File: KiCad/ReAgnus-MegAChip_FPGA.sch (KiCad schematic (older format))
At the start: 2 parts, among them U7 GW1N-UV9LQ144

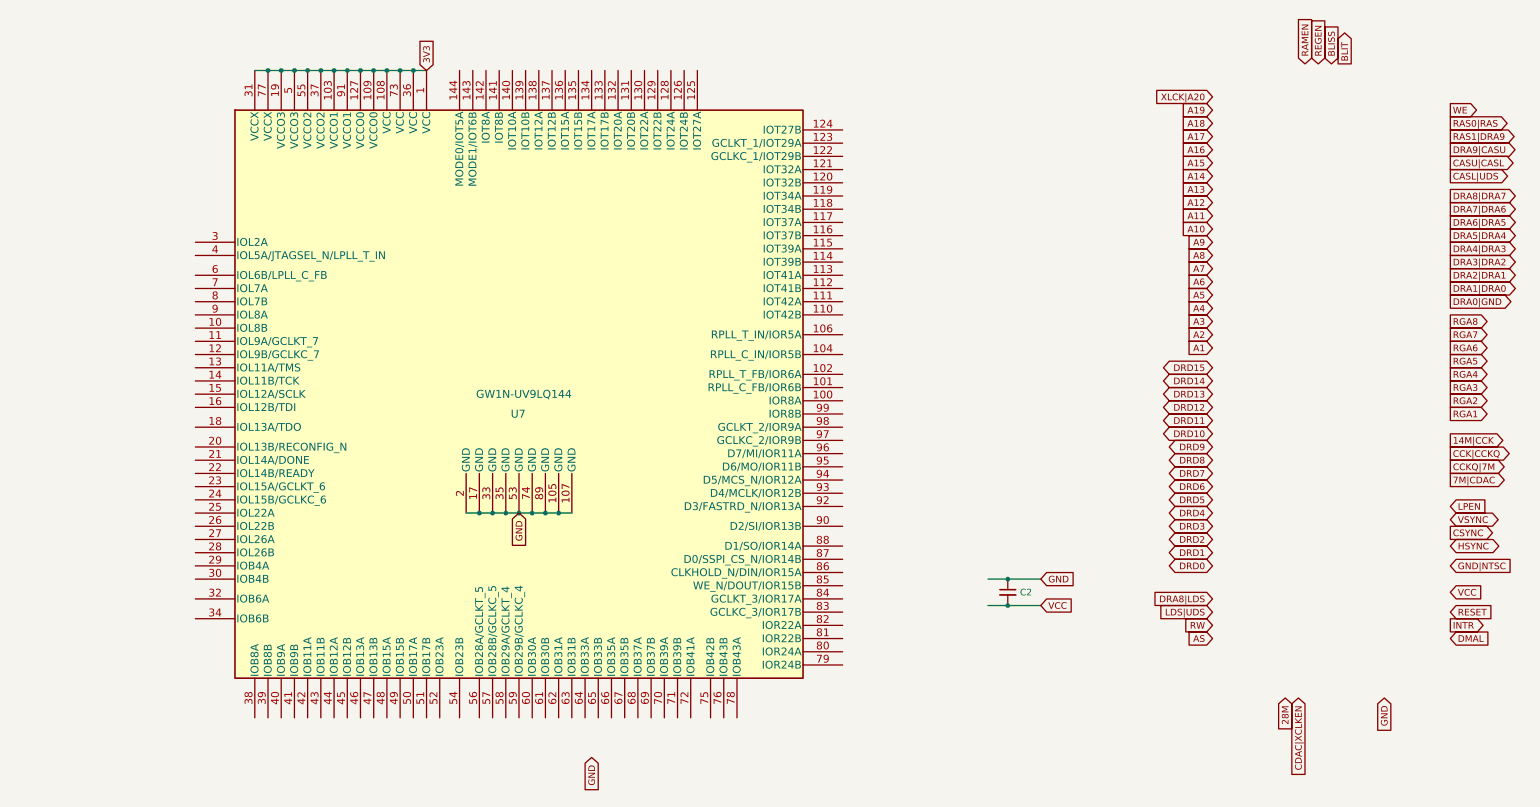
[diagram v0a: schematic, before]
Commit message: more routing and placing components
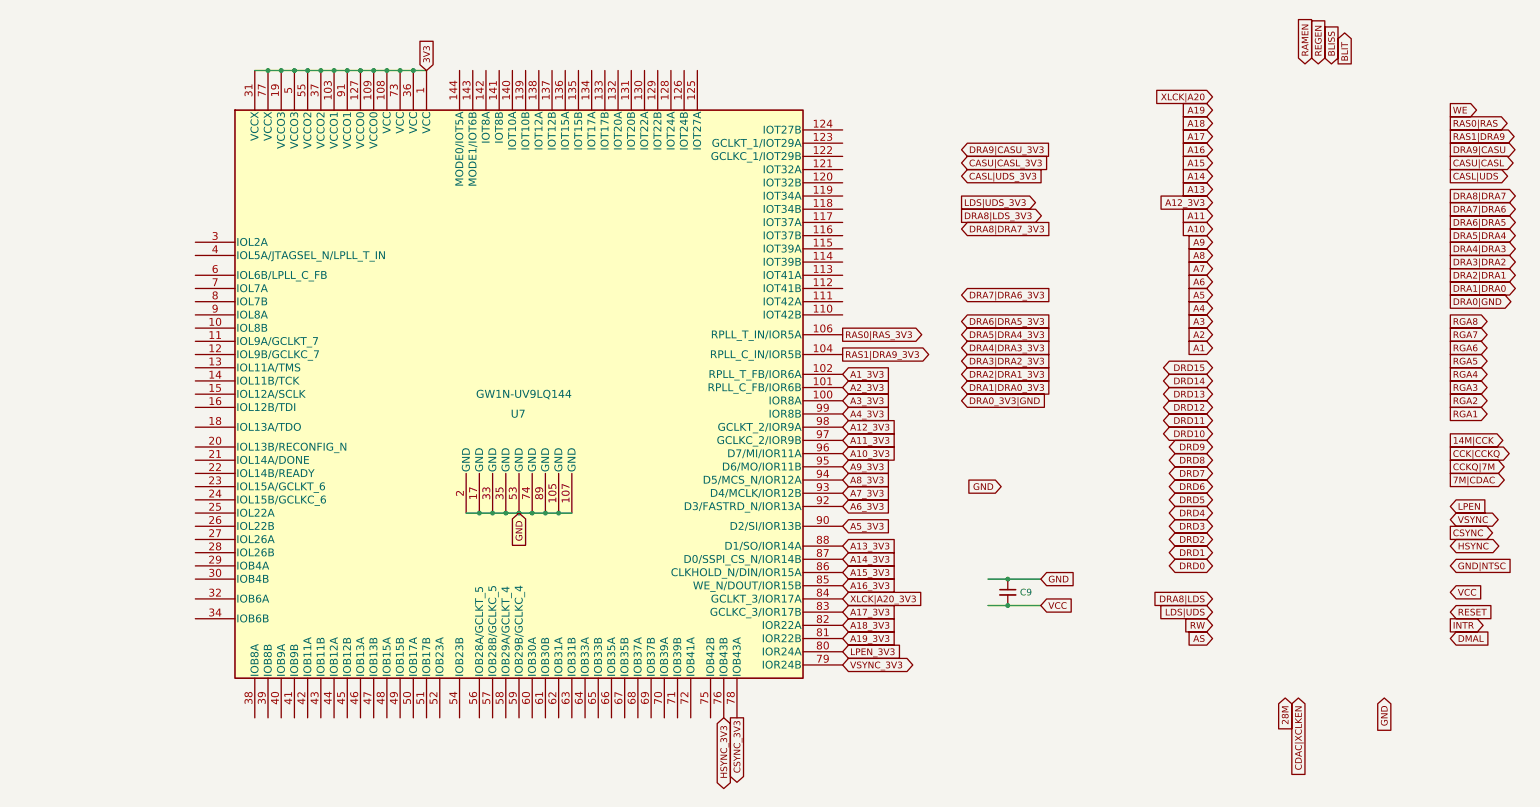
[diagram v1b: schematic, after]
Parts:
- U7: footprint Package_QFP:EQFP-144-1EP_20x20mm_P0.5mm_EP5x5mm -> Package_QFP:LQFP-144_20x20mm_P0.5mm
- renumbered C2 to C9
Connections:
- net labels added: A10_3V3, A11_3V3, A12_3V3, A13_3V3, A14_3V3, A15_3V3, A16_3V3, A17_3V3, A18_3V3, A19_3V3, A1_3V3, A2_3V3, A3_3V3, A4_3V3, A5_3V3, A6_3V3, A7_3V3, A8_3V3, A9_3V3, CASL|UDS_3V3, CASU|CASL_3V3, CSYNC_3V3, DRA0_3V3|GND, DRA1|DRA0_3V3, DRA2|DRA1_3V3, DRA3|DRA2_3V3, DRA4|DRA3_3V3, DRA5|DRA4_3V3, DRA6|DRA5_3V3, DRA7|DRA6_3V3, DRA8|DRA7_3V3, DRA8|LDS_3V3, DRA9|CASU_3V3, HSYNC_3V3, LDS|UDS_3V3, LPEN_3V3, RAS0|RAS_3V3, RAS1|DRA9_3V3, VSYNC_3V3, XLCK|A20_3V3
- net labels removed: A12
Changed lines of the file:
@@
 Comment4 ""
 $EndDescr
-Text GLabel 3900 6350 3    50   Input ~ 0
+Text GLabel 7000 4300 0    50   Input ~ 0
 GND
 Text GLabel 7300 5200 2    50   Input ~ 0
@@
 AR Path="/632F85C6" Ref="C?"  Part="1"
 AR Path="/632D3BDF/632F85C6" Ref="C?"  Part="1"
-AR Path="/632F104D/632F85C6" Ref="C2"  Part="1"
-F 0 "C2" H 7142 5100 50  0000 L CNN
+AR Path="/632F104D/632F85C6" Ref="C9"  Part="1"
+F 0 "C9" H 7142 5100 50  0000 L CNN
 F 1 "C_Small" H 7142 5055 50  0001 L CNN
 F 2 "Capacitor_SMD:C_1206_3216Metric_Pad1.42x1.75mm_HandSolder" H 7050 5100 50  0001 C CNN
@@
 F 0 "U7" H 3400 3450 60  0000 R CNN
 F 1 "GW1N-UV9LQ144" H 3750 3600 60  0000 R CNN
-F 2 "Package_QFP:EQFP-144-1EP_20x20mm_P0.5mm_EP5x5mm" H 3350 3700 60  0001 C CNN
+F 2 "Package_QFP:LQFP-144_20x20mm_P0.5mm" H 3350 3700 60  0001 C CNN
 F 3 "https://www.mouser.com/datasheet/2/1033/GW1N_series_of_FPGA_Products_Data_Sheet-1830682.pdf" H 4800 4800 60  0001 C CNN
 	1    3350 3600
@@
 A13
 Text GLabel 8600 2150 0    50   Input ~ 0
-A12
+A12_3V3
 Text GLabel 8600 2250 0    50   Input ~ 0
 A11
@@
 Text GLabel 10400 4900 2    50   Input ~ 0
 GND|NTSC
+Text GLabel 5800 5350 2    50   Input ~ 0
+A18_3V3
+Text GLabel 5800 5450 2    50   Input ~ 0
+A19_3V3
+Text GLabel 5800 5250 2    50   Input ~ 0
+A17_3V3
+Text GLabel 5800 5050 2    50   Input ~ 0
+A16_3V3
+Text GLabel 5800 4950 2    50   Input ~ 0
+A15_3V3
+Text GLabel 5800 4850 2    50   Input ~ 0
+A14_3V3
+Text GLabel 5800 4750 2    50   Input ~ 0
+A13_3V3
+Text GLabel 5800 3850 2    50   Input ~ 0
+A12_3V3
+Text GLabel 5800 3950 2    50   Input ~ 0
+A11_3V3
+Text GLabel 5800 4050 2    50   Input ~ 0
+A10_3V3
+Text GLabel 5800 4150 2    50   Input ~ 0
+A9_3V3
+Text GLabel 5800 4250 2    50   Input ~ 0
+A8_3V3
+Text GLabel 5800 4350 2    50   Input ~ 0
+A7_3V3
+Text GLabel 5800 4450 2    50   Input ~ 0
+A6_3V3
+Text GLabel 5800 4600 2    50   Input ~ 0
+A5_3V3
+Text GLabel 5800 5150 2    50   Input ~ 0
+XLCK|A20_3V3
+Text GLabel 4900 6050 3    50   BiDi ~ 0
+HSYNC_3V3
+Text GLabel 5000 6050 3    50   Output ~ 0
+CSYNC_3V3
+Text GLabel 5800 5650 2    50   BiDi ~ 0
+VSYNC_3V3
+Text GLabel 5800 5550 2    50   Input ~ 0
+LPEN_3V3
+Text GLabel 5800 3750 2    50   Input ~ 0
+A4_3V3
+Text GLabel 5800 3650 2    50   Input ~ 0
+A3_3V3
+Text GLabel 5800 3550 2    50   Input ~ 0
+A2_3V3
+Text GLabel 5800 3450 2    50   Input ~ 0
+A1_3V3
+Text GLabel 5800 3150 2    50   Output ~ 0
+RAS0|RAS_3V3
+Text GLabel 5800 3300 2    50   Output ~ 0
+RAS1|DRA9_3V3
+Text GLabel 6700 1750 2    50   Input ~ 0
+DRA9|CASU_3V3
+Text GLabel 6700 1850 2    50   Input ~ 0
+CASU|CASL_3V3
+Text GLabel 6700 1950 2    50   Input ~ 0
+CASL|UDS_3V3
+Text GLabel 6700 2150 2    50   Output ~ 0
+LDS|UDS_3V3
+Text GLabel 6700 2250 2    50   Output ~ 0
+DRA8|LDS_3V3
+Text GLabel 6700 2350 2    50   Input ~ 0
+DRA8|DRA7_3V3
+Text GLabel 6700 2850 2    50   Input ~ 0
+DRA7|DRA6_3V3
+Text GLabel 6700 3050 2    50   Input ~ 0
+DRA6|DRA5_3V3
+Text GLabel 6700 3150 2    50   Input ~ 0
+DRA5|DRA4_3V3
+Text GLabel 6700 3250 2    50   Input ~ 0
+DRA4|DRA3_3V3
+Text GLabel 6700 3350 2    50   Input ~ 0
+DRA3|DRA2_3V3
+Text GLabel 6700 3450 2    50   Input ~ 0
+DRA2|DRA1_3V3
+Text GLabel 6700 3550 2    50   Input ~ 0
+DRA1|DRA0_3V3
+Text GLabel 6700 3650 2    50   Input ~ 0
+DRA0_3V3|GND
 $EndSCHEMATC

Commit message: more routing and placing components
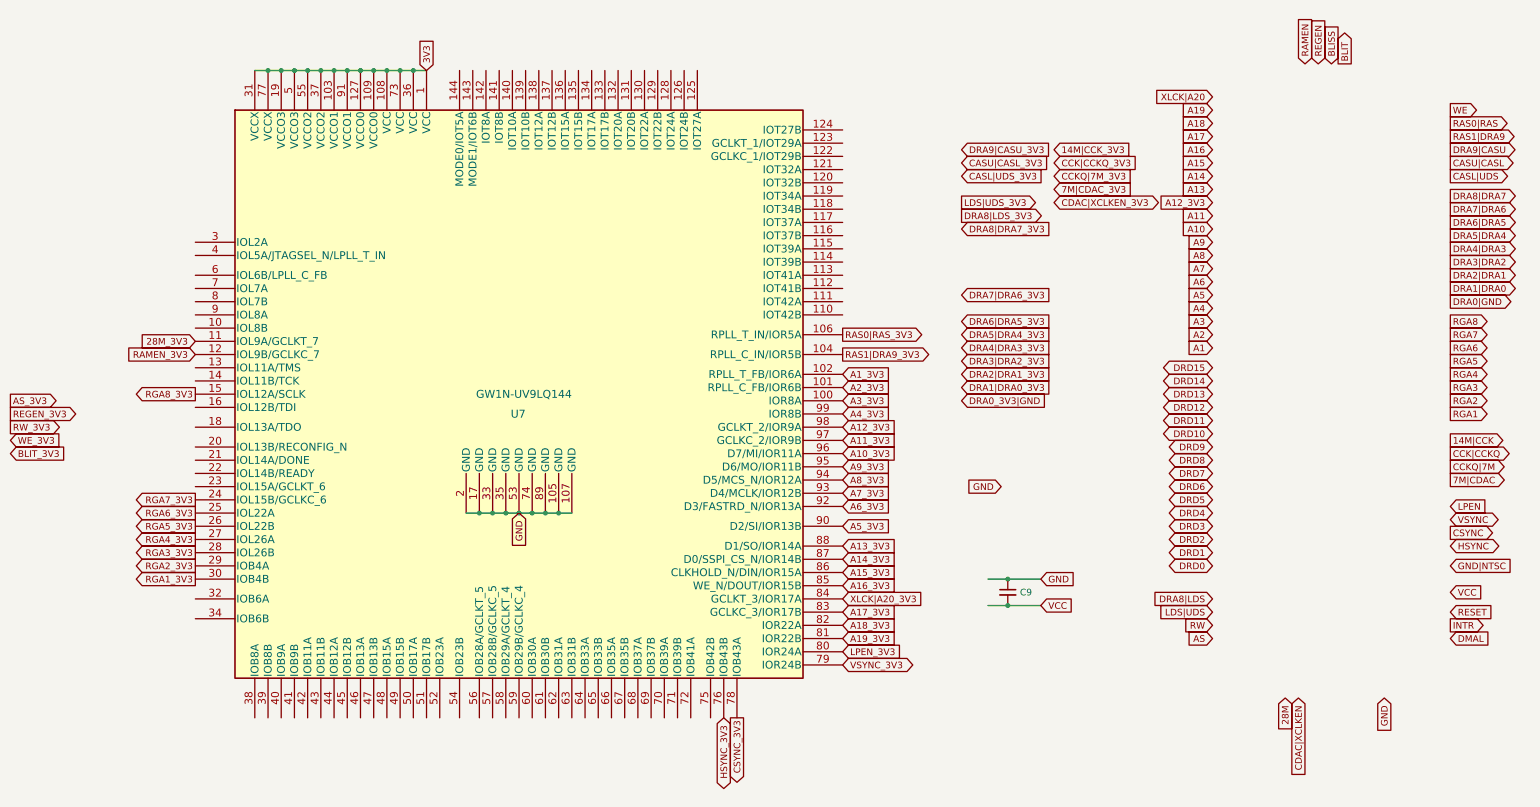
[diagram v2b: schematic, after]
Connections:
- net labels added: 14M|CCK_3V3, 28M_3V3, 7M|CDAC_3V3, AS_3V3, BLIT_3V3, CCKQ|7M_3V3, CCK|CCKQ_3V3, CDAC|XCLKEN_3V3, RAMEN_3V3, REGEN_3V3, RGA1_3V3, RGA2_3V3, RGA3_3V3, RGA4_3V3, RGA5_3V3, RGA6_3V3, RGA7_3V3, RGA8_3V3, RW_3V3, WE_3V3
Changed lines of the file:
@@
 Text GLabel 6700 3650 2    50   Input ~ 0
 DRA0_3V3|GND
+Text GLabel -500 4050 2    50   Input ~ 0
+BLIT_3V3
+Text GLabel -500 3950 2    50   Input ~ 0
+WE_3V3
+Text GLabel -500 3850 2    50   Output ~ 0
+RW_3V3
+Text GLabel -500 3750 2    50   Output ~ 0
+REGEN_3V3
+Text GLabel -500 3650 2    50   Output ~ 0
+AS_3V3
+Text GLabel 900  3300 0    50   Input ~ 0
+RAMEN_3V3
+Text GLabel 900  3200 0    50   Input ~ 0
+28M_3V3
+Text GLabel 7400 1950 2    50   Input ~ 0
+CCKQ|7M_3V3
+Text GLabel 7400 1850 2    50   Input ~ 0
+CCK|CCKQ_3V3
+Text GLabel 7400 1750 2    50   Input ~ 0
+14M|CCK_3V3
+Text GLabel 7400 2050 2    50   Input ~ 0
+7M|CDAC_3V3
+Text GLabel 7400 2150 2    50   BiDi ~ 0
+CDAC|XCLKEN_3V3
+Text GLabel 900  5000 0    50   Output ~ 0
+RGA1_3V3
+Text GLabel 900  4900 0    50   Output ~ 0
+RGA2_3V3
+Text GLabel 900  4800 0    50   Output ~ 0
+RGA3_3V3
+Text GLabel 900  4700 0    50   Output ~ 0
+RGA4_3V3
+Text GLabel 900  4600 0    50   Output ~ 0
+RGA5_3V3
+Text GLabel 900  4500 0    50   Output ~ 0
+RGA6_3V3
+Text GLabel 900  4400 0    50   Output ~ 0
+RGA7_3V3
+Text GLabel 900  3600 0    50   Output ~ 0
+RGA8_3V3
 $EndSCHEMATC
